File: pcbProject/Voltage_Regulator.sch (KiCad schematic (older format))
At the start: 4 parts, among them U1 NCP1117

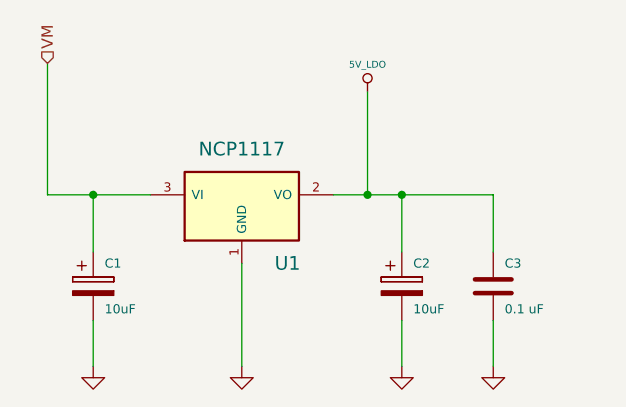
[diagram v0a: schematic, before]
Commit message: deel1routingpcb
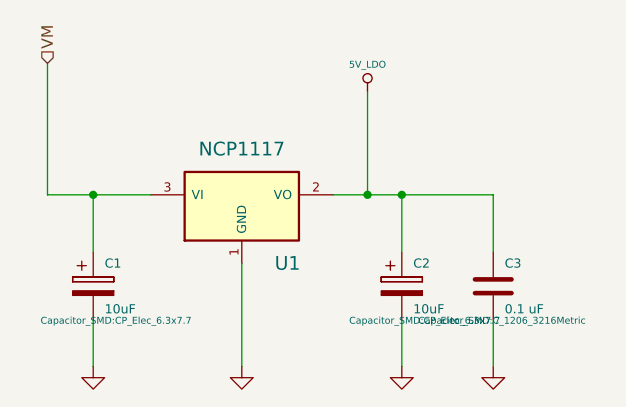
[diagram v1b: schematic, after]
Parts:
- C1, C2: footprint ~ -> Capacitor_SMD:CP_Elec_6.3x7.7
- C3: footprint ~ -> Capacitor_SMD:C_1206_3216Metric
- U1: footprint (none) -> LD1117S33CTR:SOT223
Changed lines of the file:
@@
 F 0 "C1" H 5325 4275 40  0000 L CNN
 F 1 "10uF" H 5325 4075 40  0000 L CNN
-F 2 "~" H 5375 4025 30  0000 C CNN
+F 2 "Capacitor_SMD:CP_Elec_6.3x7.7" H 5375 4025 30  0000 C CNN
 F 3 "http://images.ihscontent.net/vipimages/VipMasterIC/IC/BEYS/BEYSS04513/BEYSS04513-1.pdf" H 5275 4175 300 0001 C CNN
 F 4 "CAPACITOR, ALUMINUM ELECTROLYTIC, NON SOLID, POLARIZED, 50 V, 47 uF, SURFACE MOUNT, 3131, CHIP, ROHS COMPLIANT" H 5275 4175 60  0001 C CNN "Characteristics"
@@
 F 0 "C3" H 7075 4275 40  0000 L CNN
 F 1 "0.1 uF" H 7075 4075 40  0000 L CNN
-F 2 "~" H 7063 4025 30  0000 C CNN
+F 2 "Capacitor_SMD:C_1206_3216Metric" H 7063 4025 30  0000 C CNN
 F 3 "http://images.ihscontent.net/vipimages/VipMasterIC/IC/KEME/KEMES10043/KEMES10043-1.pdf" H 7025 4175 60  0001 C CNN
 F 4 "CAPACITOR, CERAMIC, MULTILAYER, 100 V, X7R, 0.1 uF, SURFACE MOUNT, 0805, CHIP, ROHS COMPLIANT" H 7025 4175 60  0001 C CNN "Characteristics"
@@
 F 0 "C2" H 6675 4275 40  0000 L CNN
 F 1 "10uF" H 6675 4075 40  0000 L CNN
-F 2 "~" H 6725 4025 30  0000 C CNN
+F 2 "Capacitor_SMD:CP_Elec_6.3x7.7" H 6725 4025 30  0000 C CNN
 F 3 "http://images.ihscontent.net/vipimages/VipMasterIC/IC/BEYS/BEYSS04513/BEYSS04513-1.pdf" H 6625 4175 300 0001 C CNN
 F 4 "CAPACITOR, ALUMINUM ELECTROLYTIC, NON SOLID, POLARIZED, 50 V, 47 uF, SURFACE MOUNT, 3131, CHIP, ROHS COMPLIANT" H 6625 4175 60  0001 C CNN "Characteristics"
@@
 F 0 "U1" H 6125 3575 60  0000 C CNN
 F 1 "NCP1117" H 5925 4075 60  0000 C CNN
-F 2 "" H 5925 3825 60  0001 C CNN
+F 2 "LD1117S33CTR:SOT223" H 5925 3825 60  0001 C CNN
 F 3 "http://www.st.com/st-web-ui/static/active/en/resource/technical/document/datasheet/CD00000544.pdf" H 5925 3825 60  0001 C CNN
 F 4 "5 V FIXED POSITIVE LDO REGULATOR, 1.2 V DROPOUT, PDSO3, ROHS COMPLIANT, SOT-223, 4 PIN" H 5925 3825 60  0001 C CNN "Characteristics"
